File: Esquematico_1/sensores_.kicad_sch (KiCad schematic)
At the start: 10 parts, among them IC1 MAX-M10M-00B, U1 ICM-42688-P, U3 Mag, U4 BMP388

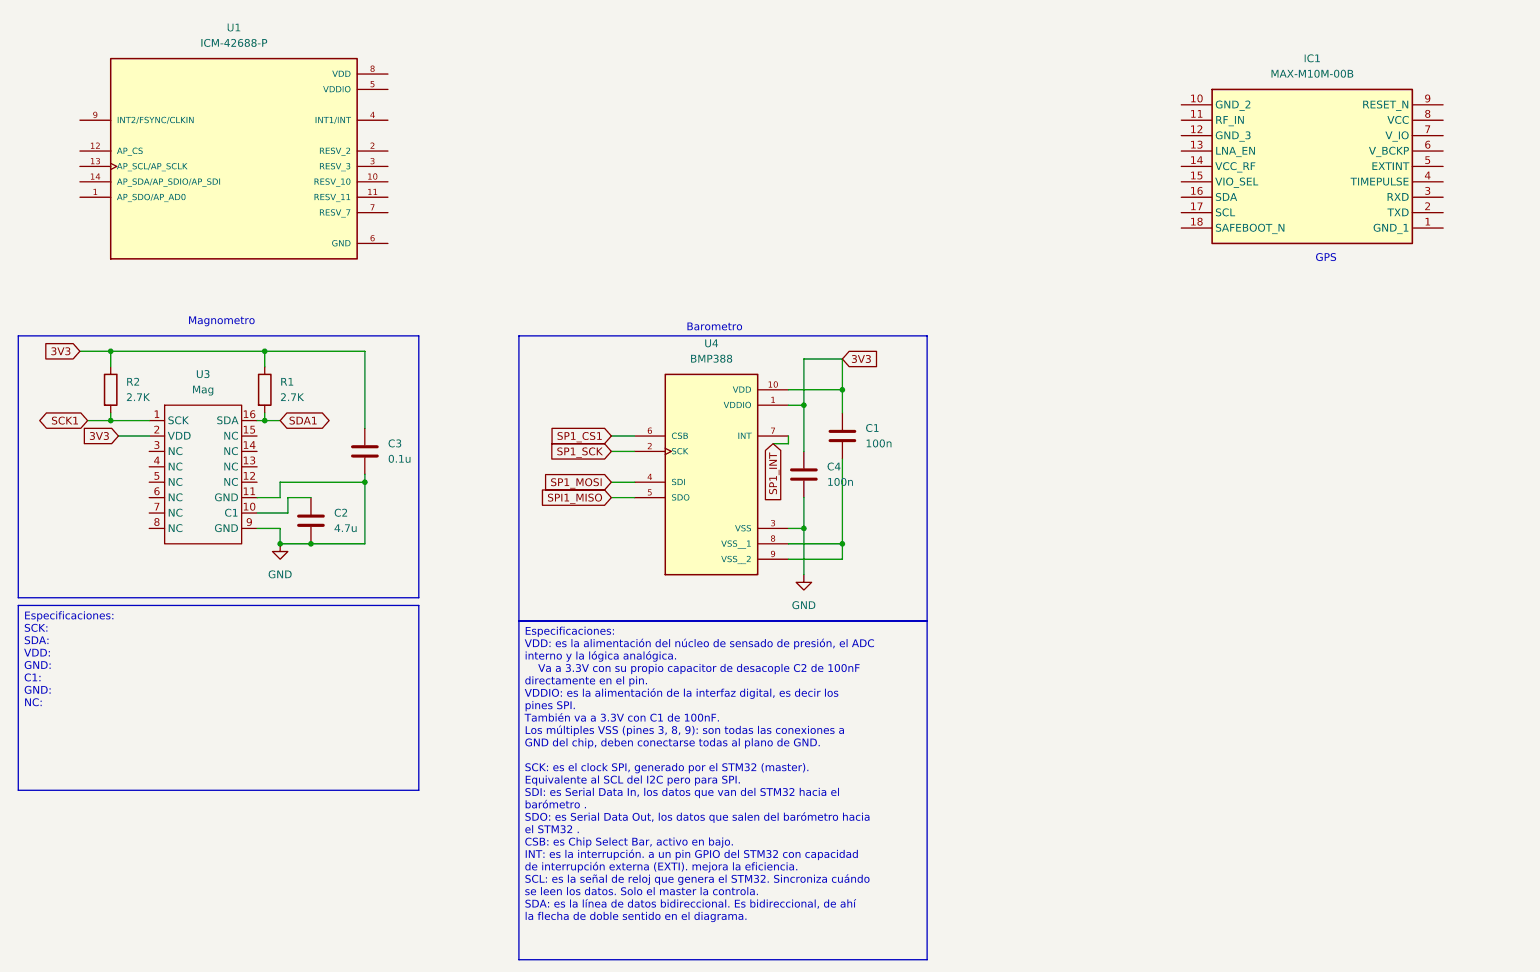
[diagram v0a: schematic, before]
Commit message: Imu
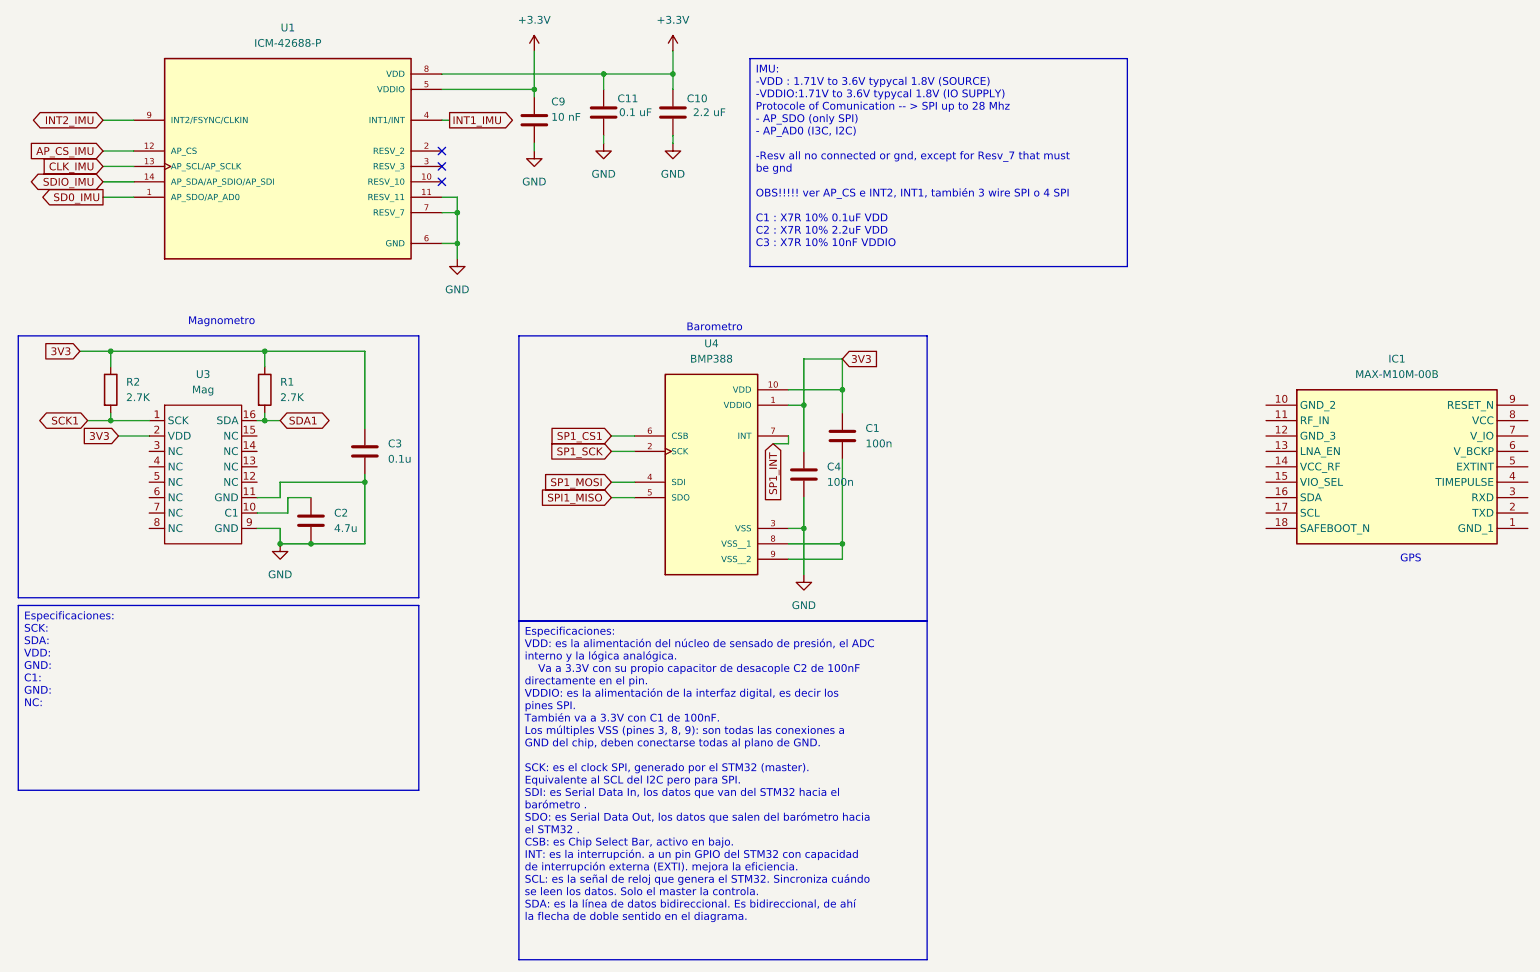
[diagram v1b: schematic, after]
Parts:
- added C10: 2.2 uF, symbol Device:C
- added C11: 0.1 uF, symbol Device:C
- added C9: 10 nF, symbol Device:C
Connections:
- net GND: now also U1.11 (RESV_11), U1.6 (GND), U1.7 (RESV_7), C10.2, C11.2, C9.2
- net SD0_IMU: now reaches U1.1 (AP_SDO/AP_AD0)
- net AP_CS_IMU: now reaches U1.12 (AP_CS)
- net CLK_IMU: now reaches U1.13 (AP_SCL/AP_SCLK)
- net SDIO_IMU: now reaches U1.14 (AP_SDA/AP_SDIO/AP_SDI)
- net INT1_IMU: now reaches U1.4 (INT1/INT)
- net +3.3V: now reaches U1.5 (VDDIO)
- net +3.3V: now also U1.8 (VDD), C10.1, C11.1, C9.1
- net INT2_IMU: now reaches U1.9 (INT2/FSYNC/CLKIN)
- no-connect marks 0 -> 3
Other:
- moved on the sheet: IC1, U1
